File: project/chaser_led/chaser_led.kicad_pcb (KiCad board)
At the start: 2 copper layers, 25 parts, among them P1 pwr, U1 NE555, U2 4017

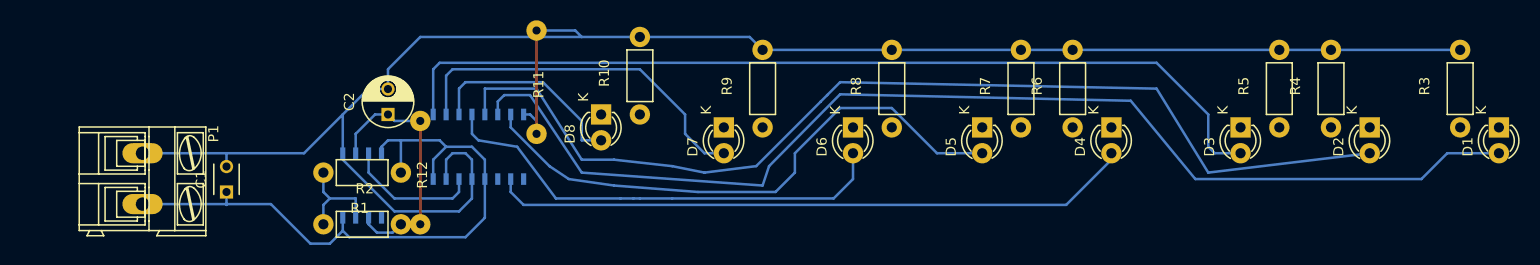
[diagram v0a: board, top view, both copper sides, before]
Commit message: a
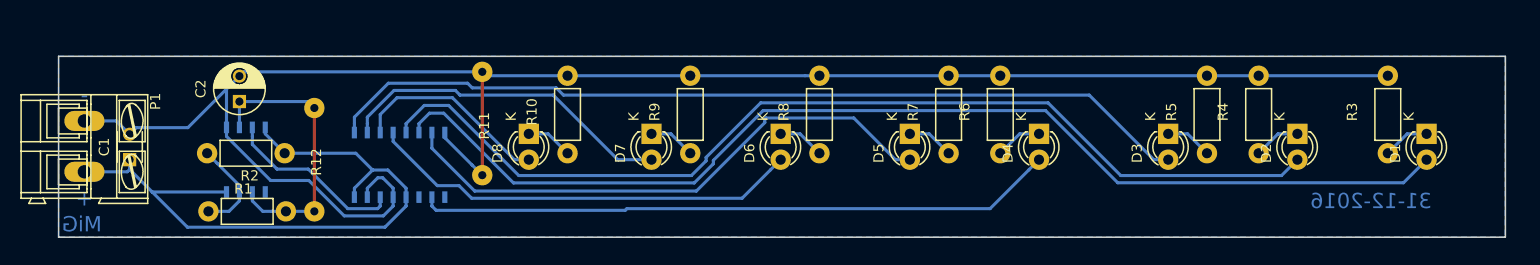
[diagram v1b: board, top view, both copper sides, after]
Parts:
- moved C2 14.7 mm to (106.7, 101.0)
- moved U1 11.7 mm to (107.3, 106.7)
- moved R1 11.6 mm to (111.1, 106.0)
- moved R2 11.4 mm to (103.6, 111.8)
- moved R12 10.5 mm to (114.0, 111.8)
- moved C1 10.0 mm to (95.9, 106.7)
- moved R10 8.07 mm to (138.9, 106.0)
- moved U2 7.95 mm to (122.4, 107.2)
- moved R9 7.55 mm to (151.0, 106.0)
- moved R3 7.55 mm to (219.6, 106.0)
- moved R4 7.55 mm to (206.9, 106.0)
- moved R5 7.55 mm to (201.8, 106.0)
- moved R6 7.55 mm to (181.5, 106.0)
- moved R7 7.55 mm to (176.4, 106.0)
- moved R8 7.55 mm to (163.7, 106.0)
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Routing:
- net GND: track 183.5 -> 178.0 mm
- net Net-(U1-Pad3): track 13.4 -> 18.2 mm
- net Net-(D8-Pad1): track 0.00 -> 4.60 mm
- net Net-(D6-Pad1): track 0.00 -> 4.60 mm
- net Net-(D5-Pad1): track 0.00 -> 4.60 mm
- net Net-(D4-Pad1): track 0.00 -> 4.60 mm
- net Net-(D3-Pad1): track 0.00 -> 4.60 mm
- net Net-(D2-Pad1): track 0.00 -> 4.60 mm
- net Net-(D1-Pad1): track 0.00 -> 4.60 mm
- net Net-(D7-Pad1): track 0.00 -> 4.60 mm
- net Net-(D3-Pad2): track 89.6 -> 86.0 mm
- net Net-(D1-Pad2): track 113.1 -> 110.2 mm
- net Net-(D2-Pad2): track 101.7 -> 98.9 mm
- net Net-(D6-Pad2): track 45.6 -> 42.9 mm
- net Net-(D7-Pad2): track 35.9 -> 33.4 mm
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- added copper zone on B.Cu, net (none)
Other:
- board outline added: 142.2 x 17.8 mm
- net class Default: clearance 0.2 -> 0.4064; trace_width 0.25 -> 0.254
- rule trace_clearance: 0.2 -> 0.4064
- board text added: "+"
- board text added: "-"
- board text added: "31-12-2016"
- board text added: "MiG"
